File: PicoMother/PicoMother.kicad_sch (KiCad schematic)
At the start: 20 parts, among them J8 M20-9980345, J9 USB_C, U5 ATmega8U2-A, Y4 Crystal_GND24

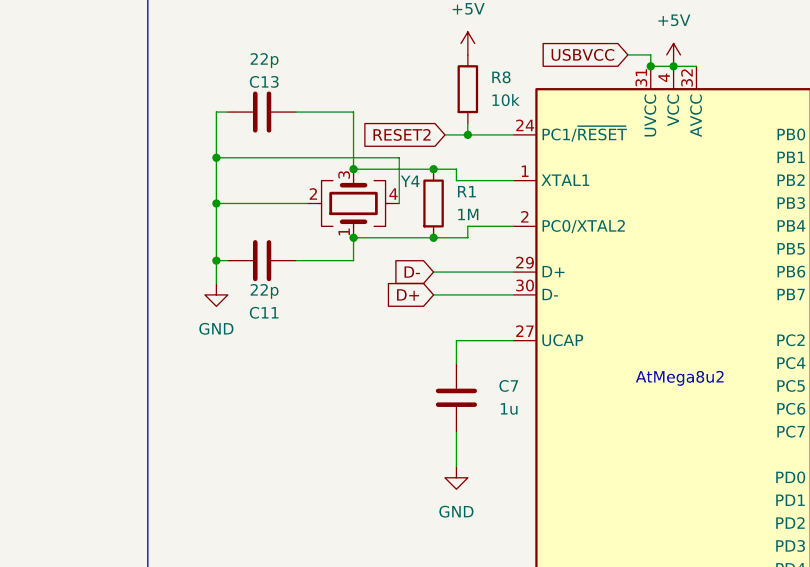
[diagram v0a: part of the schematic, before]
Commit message: Correction inversion D+ D-
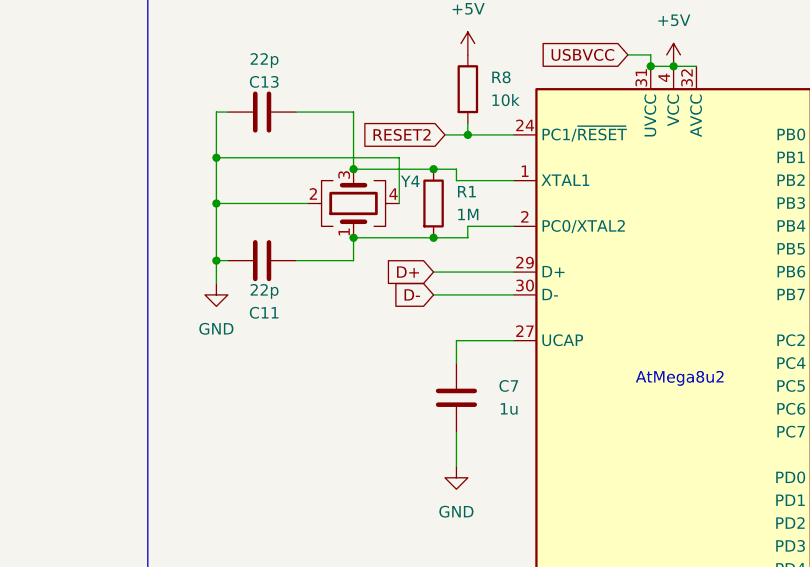
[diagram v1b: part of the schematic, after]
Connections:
- net D+: now also U5.29 (D+); no longer U5.30 (D-)
- net D-: now also U5.30 (D-); no longer U5.29 (D+)
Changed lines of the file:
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@@
 		)
 	)
-	(global_label "D-"
+	(global_label "D+"
 		(shape input)
 		(at 146.05 106.68 180)
@@
 		)
 	)
-	(global_label "D+"
+	(global_label "D-"
 		(shape input)
 		(at 146.05 109.22 180)
